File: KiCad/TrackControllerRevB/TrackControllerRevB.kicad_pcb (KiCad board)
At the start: 2 copper layers, 130 x 60 mm, 24 parts, among them J1 DE9_Plug_MountingHoles, J3 Barrel_Jack_Switch, SW1 SW_Push, SW2 SW_Push, SW3 SW_Push, SW4 SW_Push, U1 TXS0108EPW

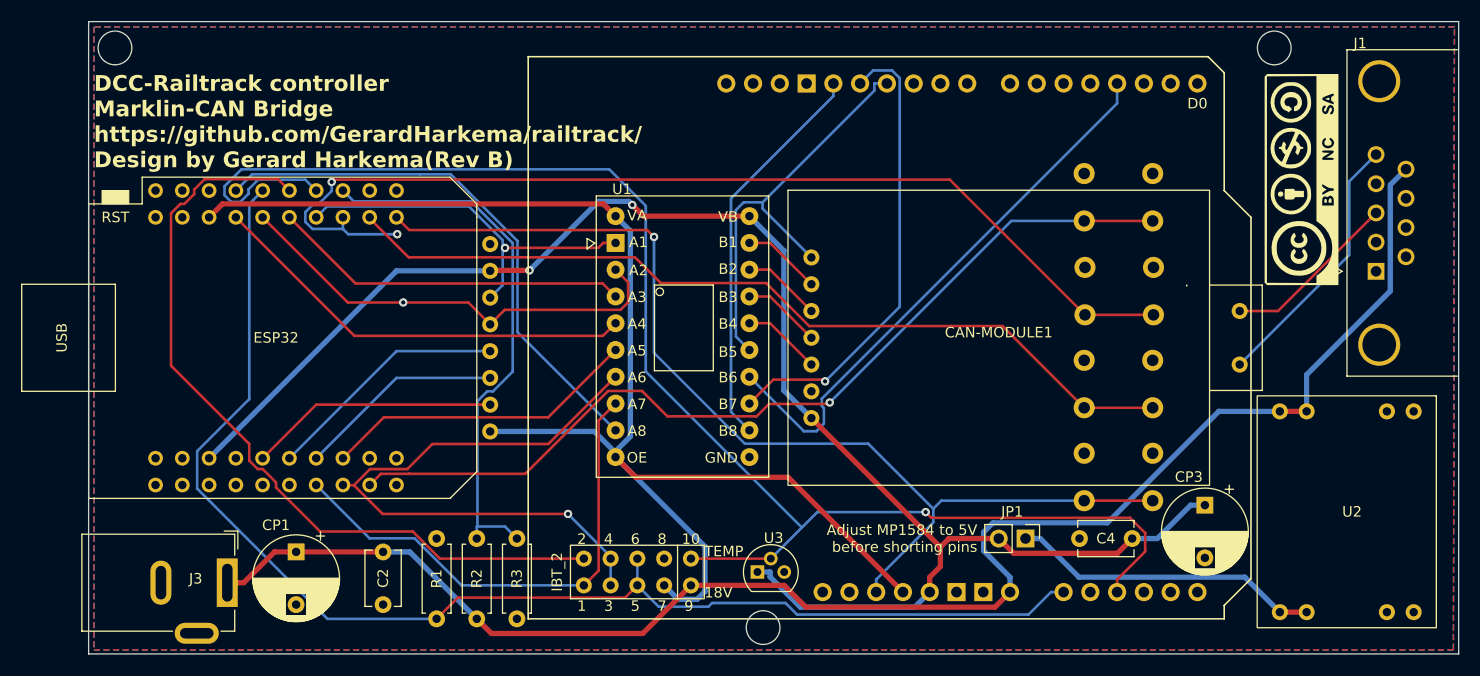
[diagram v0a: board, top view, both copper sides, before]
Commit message: 2040514
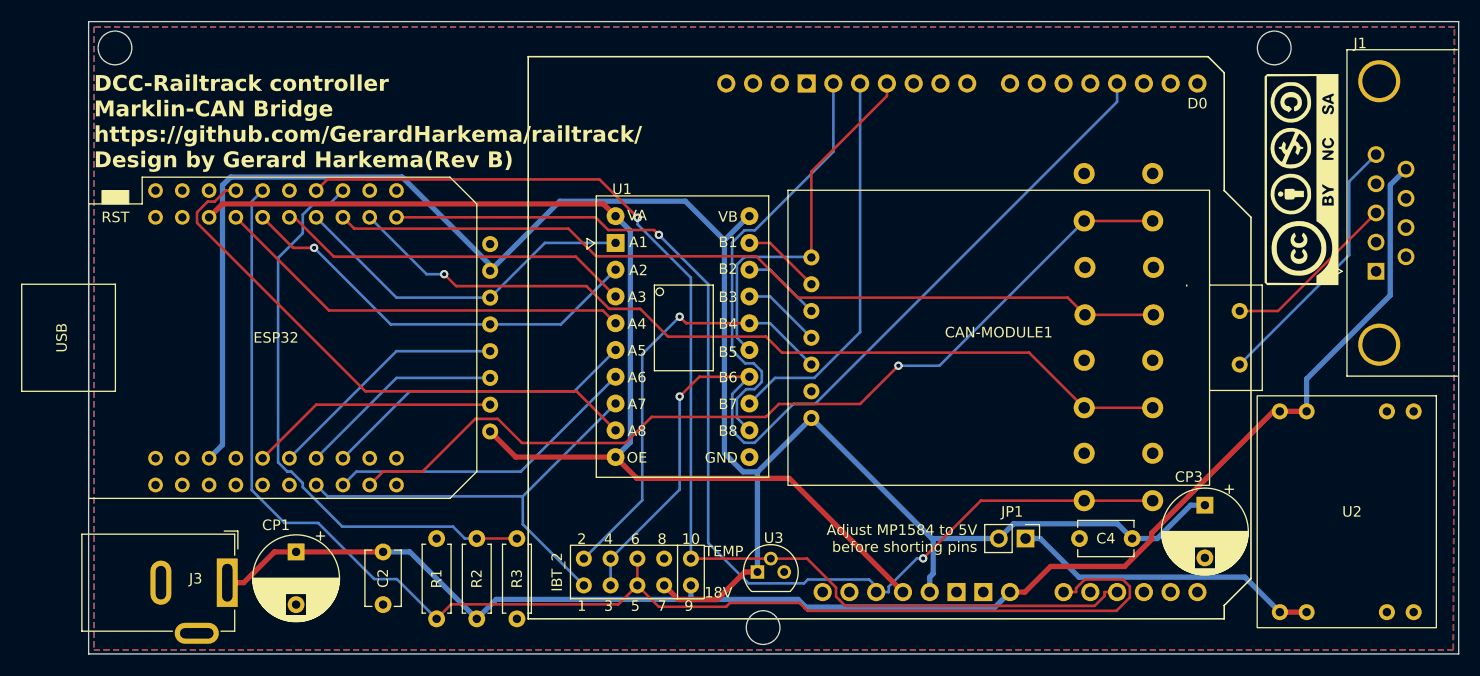
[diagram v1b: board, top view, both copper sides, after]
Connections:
- net /CAN-CS* renamed /CAN-CS*/TRACK-PULSE-L
- CAN-MODULE1 pad 5: /CAN-CS-TTL* -> /CAN-CS*/TRACK-PULSE-L-TTL
- IBT_2 pad 2: /TRACK-PULSE-L -> /CAN-CS*/TRACK-PULSE-L-TTL
- IBT_2 pad 3: /TRACK-POWER-ENABLE -> /TRACK-ENABLE-TTL
- IBT_2 pad 4: /TRACK-POWER-ENABLE -> /TRACK-ENABLE-TTL
- IBT_2 pad 7: /3V3 -> /VCC
- U1 pad 16: /CAN-CS-TTL* -> /CAN-CS*/TRACK-PULSE-L-TTL
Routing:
- net /TRACK-PULSE-L: track 75.7 -> 0.00 mm
- net /CAN-CS*/TRACK-PULSE-L-TTL: track 0.00 -> 41.1 mm, vias 0 -> 1
- net /VCC: track 152.0 -> 186.9 mm, vias 2 -> 0
- net /TRACK-ENABLE-TTL: track 53.5 -> 86.0 mm, vias 0 -> 1
- net /TEMP: track 142.6 -> 110.5 mm
- net /TRACK-POWER-ENABLE: track 60.0 -> 30.1 mm, vias 1 -> 0
- net /3V3: track 129.9 -> 109.1 mm
- net /SPARE-SWITCH-1: track 98.8 -> 80.7 mm, vias 2 -> 0
- net /TRACK-PULSE-H-TTL: track 44.5 -> 36.9 mm, vias 1 -> 0
- net /CAN-CS-TTL*: track 7.50 -> 0.00 mm
- net /18V: track 151.0 -> 143.6 mm
- net /IS: track 124.4 -> 131.2 mm
- net /RESET*: track 100.1 -> 105.6 mm, vias 1 -> 2
- net /CAN-INT*/TRACK-PROG-POWER-ENABLE-TTL: track 40.7 -> 35.5 mm
- net /TRACK-PULSE-H: track 47.8 -> 43.4 mm
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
